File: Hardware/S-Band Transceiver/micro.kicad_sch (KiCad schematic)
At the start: 46 parts, among them J3 AVR-UPDI-6, J4 USB_C_Receptacle_USB2.0_16P, SW1 SW_Push, U2 AVR128DA48x-xPT, U3 ADS1118IDGS, U4 FT231XQ

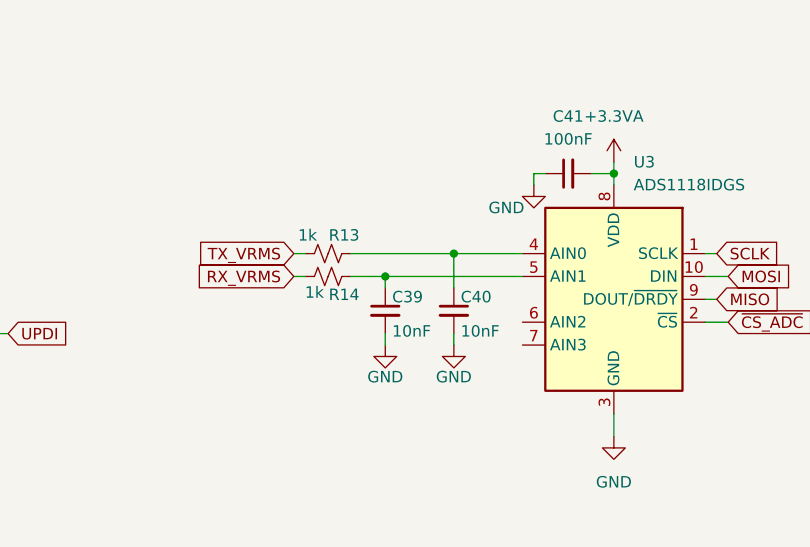
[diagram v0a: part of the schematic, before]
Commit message: updating values
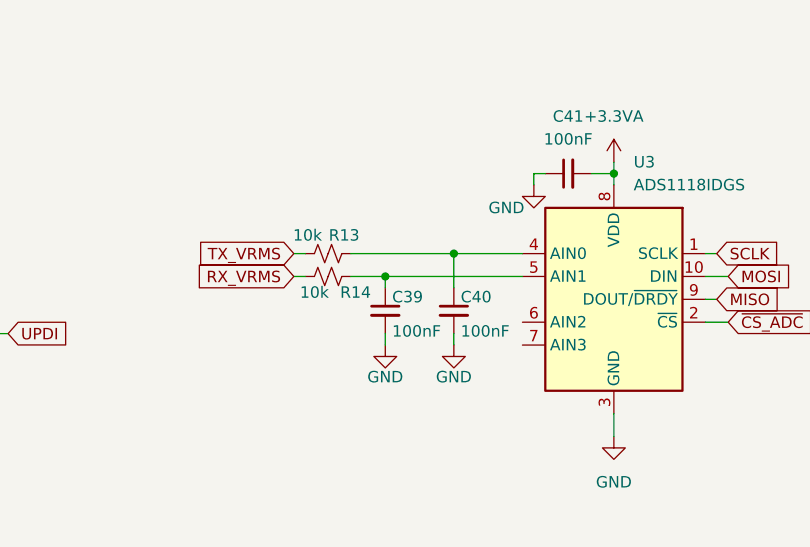
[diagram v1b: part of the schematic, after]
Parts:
- C39, C40: value 10nF -> 100nF
- R13, R14: value 1k -> 10k
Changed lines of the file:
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@@
 		(dnp no)
 		(property "Reference" "R14"
-			(at 90.678 158.242 90)
+			(at 91.948 157.988 90)
 			(effects
 				(font
@@
 			)
 		)
-		(property "Value" "1k"
+		(property "Value" "10k"
 			(at 87.376 157.988 90)
 			(effects
@@
 			)
 		)
-		(property "Value" "1k"
+		(property "Value" "10k"
 			(at 86.614 151.638 90)
 			(effects
@@
 			)
 		)
-		(property "Value" "10nF"
+		(property "Value" "100nF"
 			(at 103.632 162.306 0)
 			(effects
@@
 			)
 		)
-		(property "Value" "10nF"
+		(property "Value" "100nF"
 			(at 96.012 162.306 0)
 			(effects
